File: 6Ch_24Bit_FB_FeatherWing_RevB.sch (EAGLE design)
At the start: 19 parts, among them IC1 TPS76925, J1 CON_PTSM_SOCKET-4-PTH-VERT, J2 CON_PTSM_SOCKET-4-PTH-VERT, J3 CON_PTSM_SOCKET-4-PTH-VERT, J4 CON_PTSM_SOCKET-4-PTH-VERT, J5 CON_PTSM_SOCKET-4-PTH-VERT, J6 CON_PTSM_SOCKET-4-PTH-VERT, U1 AD7794

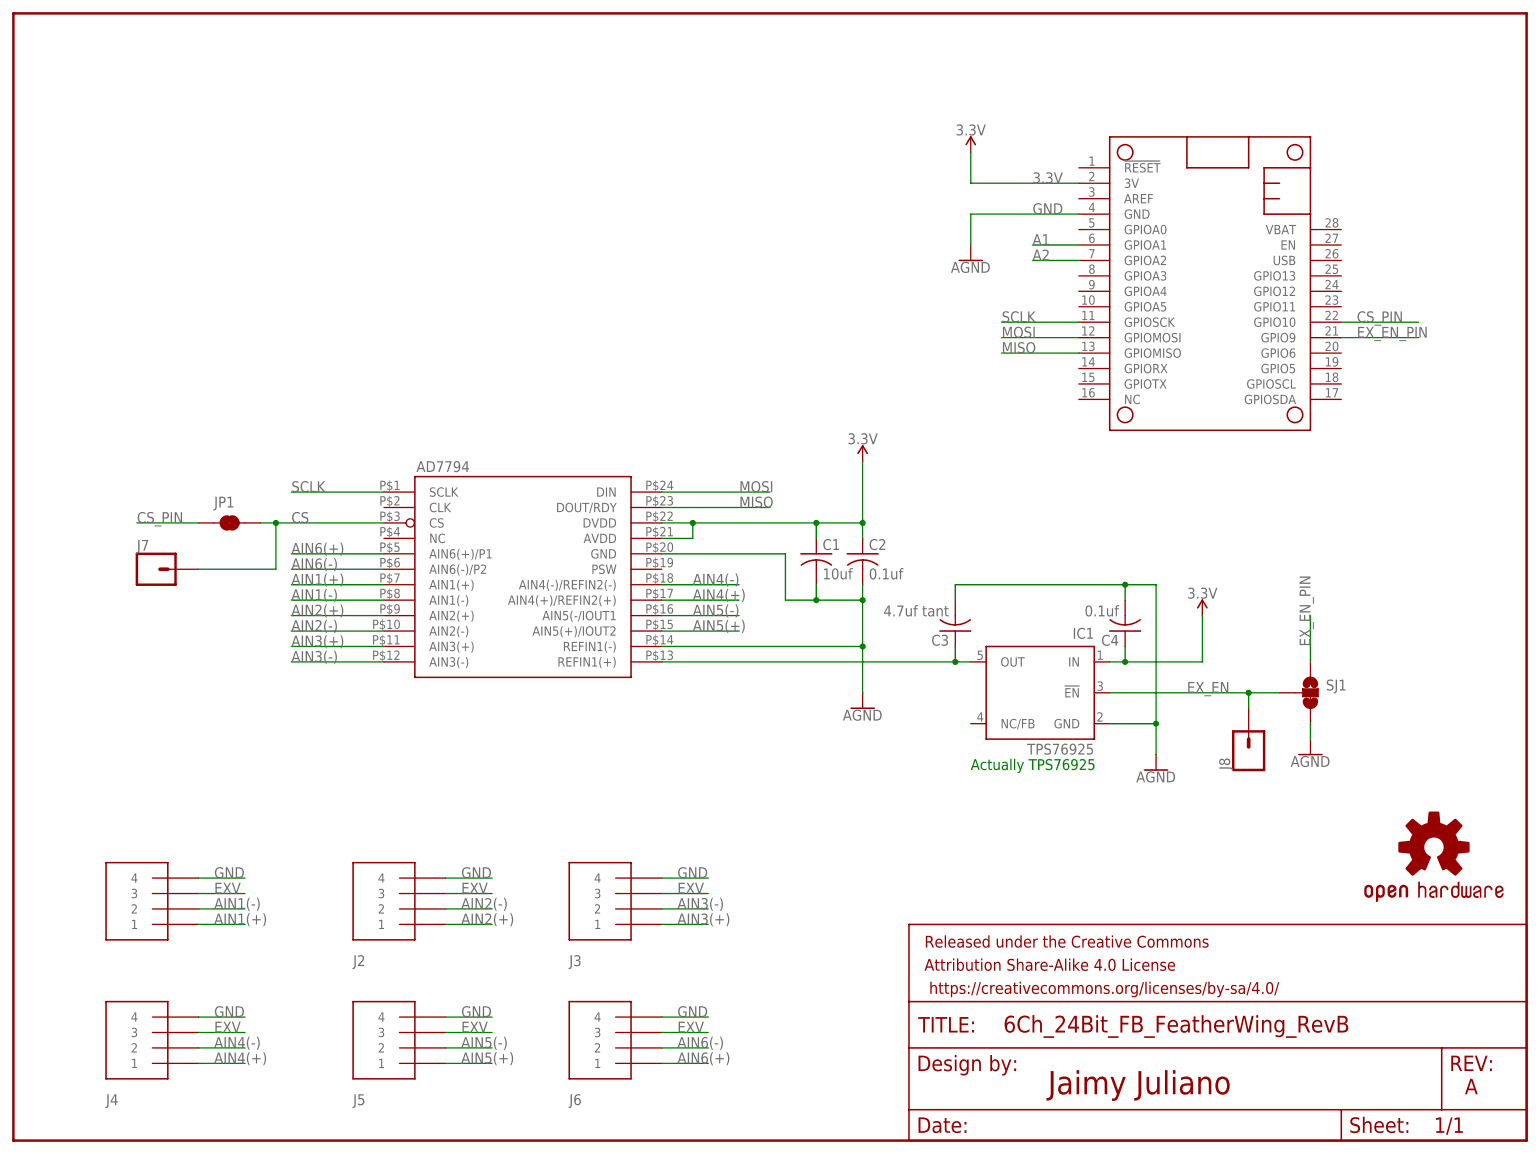
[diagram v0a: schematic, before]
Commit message: Updated to current hardware version
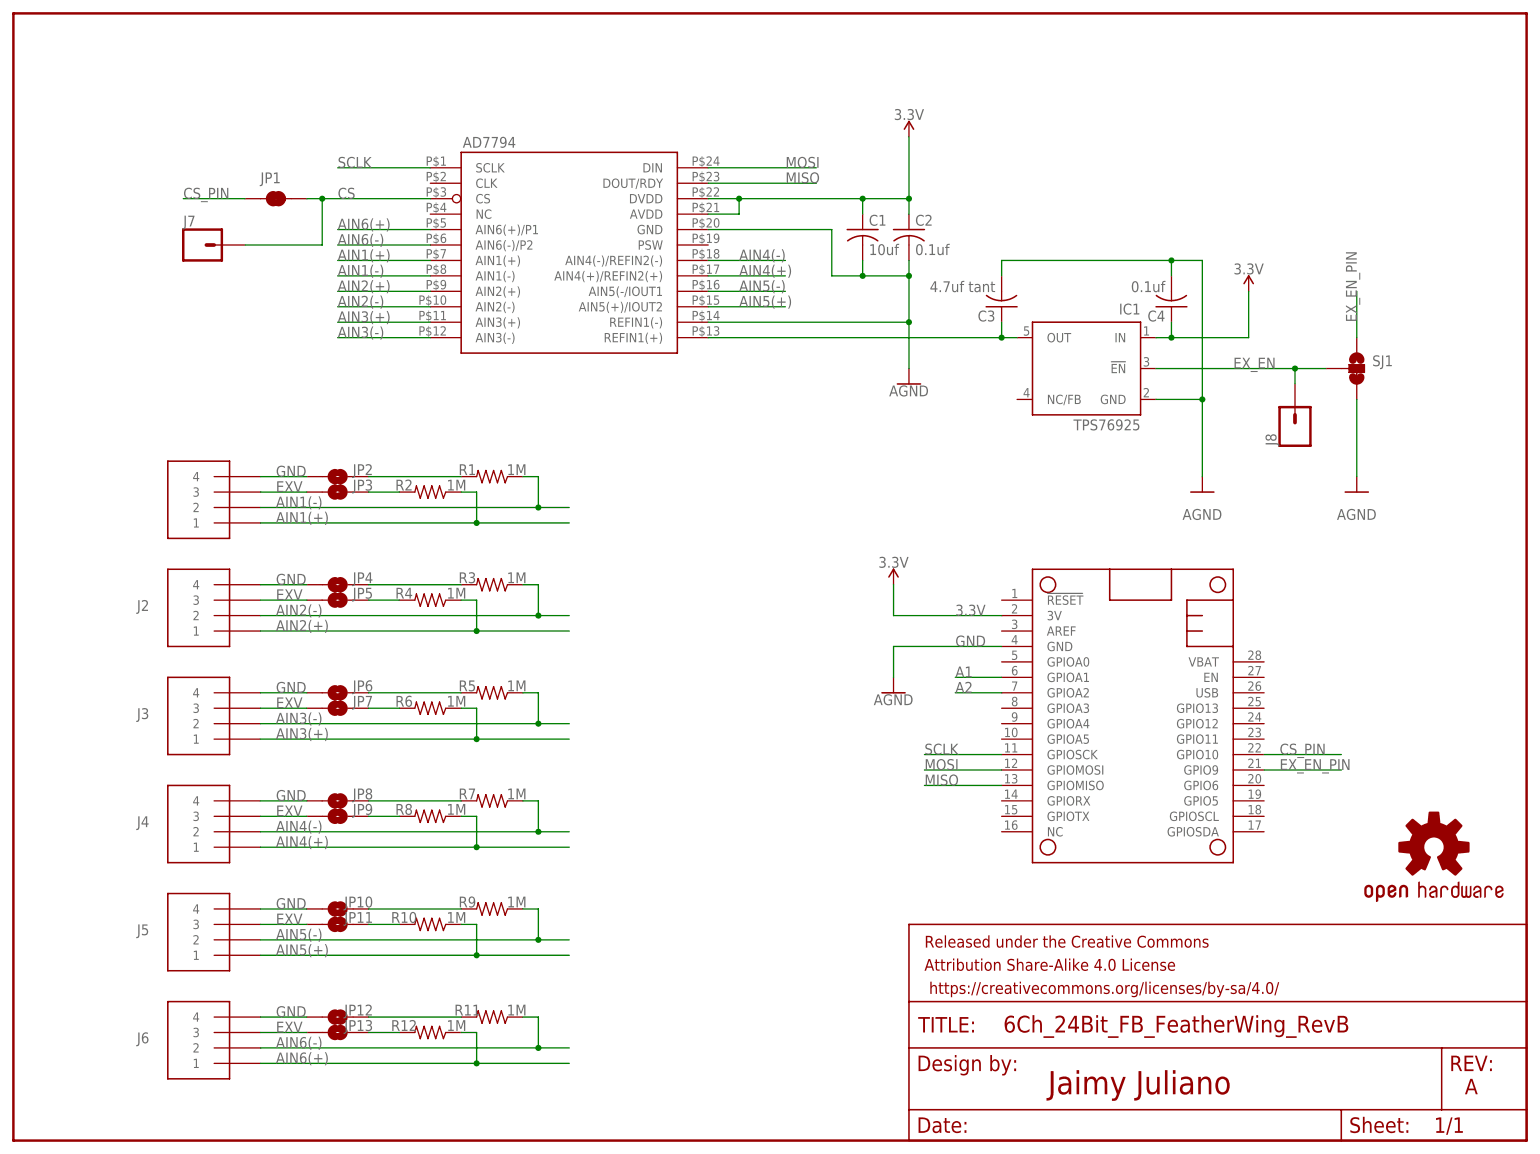
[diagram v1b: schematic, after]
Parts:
- added JP10, JP11, JP12, JP13, JP2, JP3, JP4, JP5, JP6, JP7, JP8, JP9: JUMPER-SMT_2_NO_SILK, SparkFun-Jumpers:JUMPER-SMT_2_NO_SILK
- added R1, R10, R11, R12, R2, R3, R4, R5, R6, R7, R8, R9: 1M, SparkFun-Resistors:1MOHM-0603-1/4W-5%
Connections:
- new net N$1: JP3.1, R2.2
- new net N$10: JP10.1, R9.2
- new net N$11: JP13.1, R12.2
- new net N$12: JP12.1, R11.2
- new net N$2: JP2.1, R1.2
- new net N$3: JP5.1, R4.2
- new net N$4: JP4.1, R3.2
- new net N$5: JP7.1, R6.2
- new net N$6: JP6.1, R5.2
- new net N$7: JP9.1, R8.2
- new net N$8: JP8.1, R7.2
- new net N$9: JP11.1, R10.2
- net AIN1(+): now also R2.1
- net AIN1(-): now also R1.1
- net AIN2(+): now also R4.1
- net AIN2(-): now also R3.1
- net AIN3(+): now also R6.1
- net AIN3(-): now also R5.1
- net AIN4(+): now also R8.1
- net AIN4(-): now also R7.1
- net AIN5(+): now also R10.1
- net AIN5(-): now also R9.1
- net AIN6(+): now also R12.1
- net AIN6(-): now also R11.1
- net EXV: now also JP11.2, JP13.2, JP3.2, JP5.2, JP7.2, JP9.2
- net GND: now also JP10.2, JP12.2, JP2.2, JP4.2, JP6.2, JP8.2
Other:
- note removed: "Actually TPS76925"
- moved on the sheet: C1, C2, C3, C4, IC1, J2, J3, J4, J5, J6, J7, J8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
